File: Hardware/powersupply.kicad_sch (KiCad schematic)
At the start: 34 parts, among them J4 USB_C_Receptacle_USB2.0_16P, J8 Conn_01x02_Pin, Q1 Dual_NMOS_8205A, Q2 DMG2305UX, U2 RT6150A, U3 DW01A, U6 TP4056, U9 XC6220B181MR

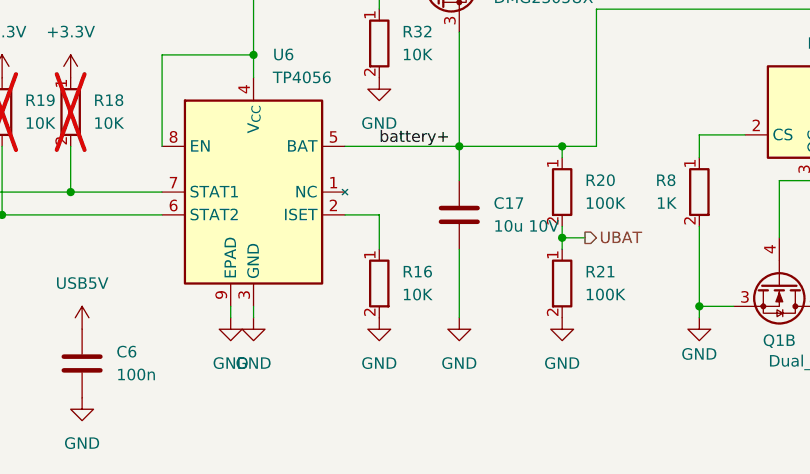
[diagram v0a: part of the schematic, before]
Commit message: mqtt und oled implementiert wip
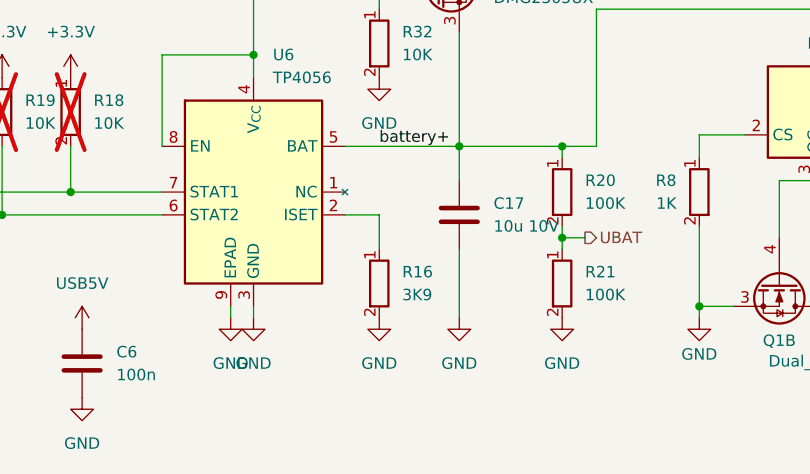
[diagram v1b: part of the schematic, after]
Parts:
- removed R16: 10K, Resistor_SMD:R_0603_1608Metric, symbol Resistor_E12_0603:Resistor 10K
- added R16: 3K9, Resistor_SMD:R_0603_1608Metric, symbol Resistor_E12_0603:Resistor 3K9
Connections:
- net GND: now also R16.2
- net at U6.2 (ISET): now also R16.1
